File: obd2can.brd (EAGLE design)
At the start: 39.7 x 29.1 mm, 21 parts, among them Q1 16MHz, SW1 6X3.5_TACT, SW3 6X3.5_TACT, U2 SN65HVD235DR, U3 STM32F030XTSSOP20, U4 MCP1700, X1 RJ45_RIGHT_ANGLEMOLEX_95001-2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

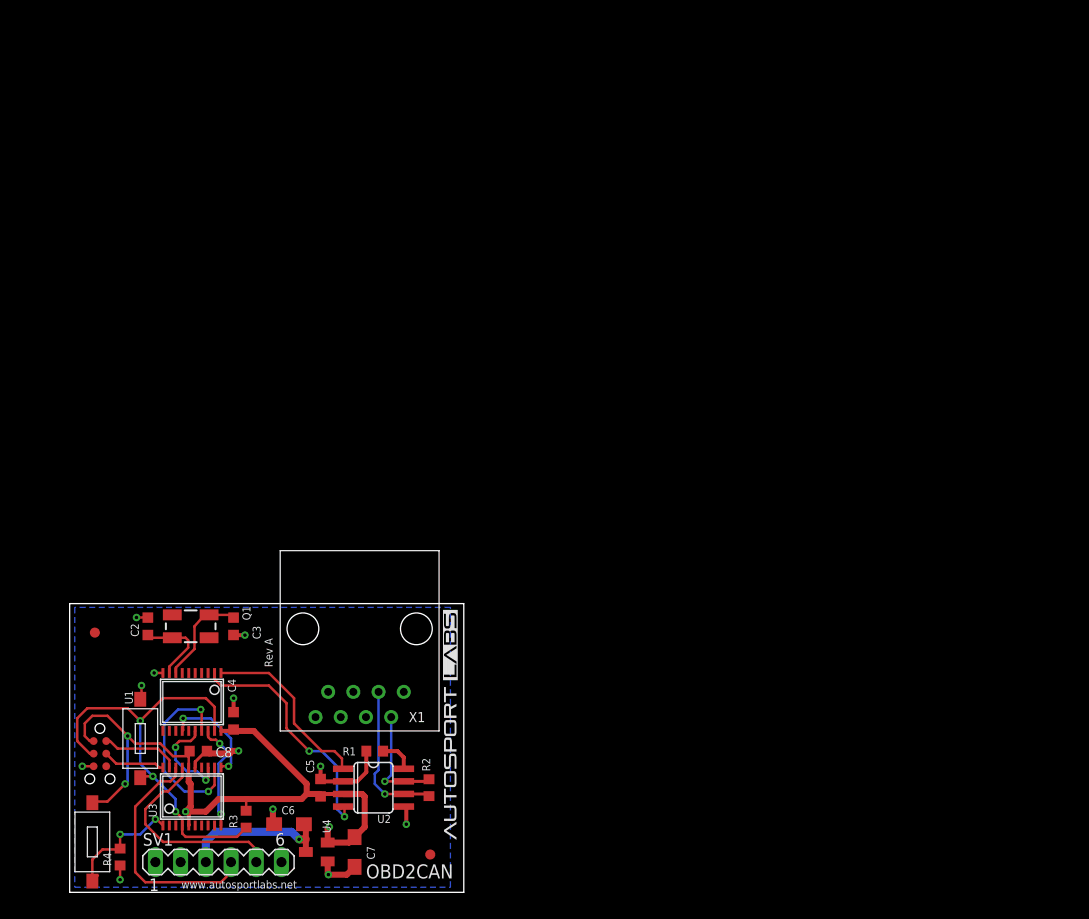
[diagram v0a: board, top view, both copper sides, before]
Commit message: OBD2CAN WIP
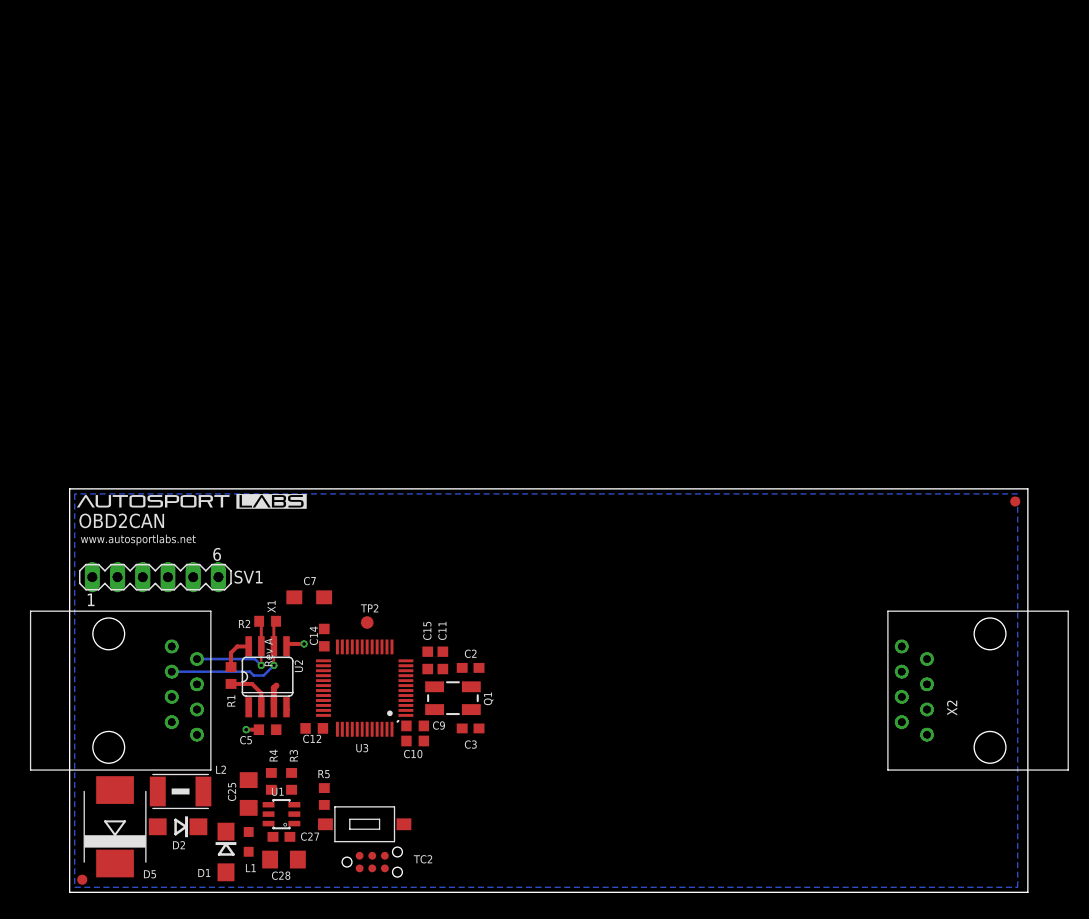
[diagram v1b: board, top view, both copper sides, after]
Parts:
- removed C4: 0.1uF, rcl:C0603K
- removed C6: 10uF, rcl:SMC_A
- removed C8: 0.1uf, rcl:C0603K
- removed SW1, SW3: 6X3.5_TACT, tactile_switch:TACT_6X3.5
- removed TC1: TC2030-IDC-NL, TagConnect:TC2030-IDC-NL
- removed U4: MCP1700, mcp1700:SOT-23
- added C10: 1uf, rcl:C0603K
- added C11: 0.01uf, rcl:C0603K
- added C12, C15: 4.7uf, rcl:C0603K
- added C14, C9: 0.1uf, rcl:C0603K
- added C25, C28: 22uF, rcl:C1206
- added C27: 10nF, rcl:C0603
- added D1: SCHOTTKY, smt_diodes:SMA
- added D2: 400V 1A, smt_diodes:SMA
- added D5: (no value), diode:SMC
- added L1: 4.7uH, rcl:L2012C
- added L2: (no value), wuerth-elektronik:1812
- added R5: 4.7K, rcl:R0603
- added SW2: 6X3.5_TACT, tactile_switch:TACT_6X3.5
- added TC2: TC2030-IDC-NL, TagConnect:TC2030-IDC-NL
- added TP2: TPB1,27, testpad:B1,27
- added X2: RJ45_RIGHT_ANGLEMOLEX_95001-2881, FCI_RJ12:RJ45_RIGHT_ANGLE_MOLEX_95001-2881
- C2, C3: value 22pF -> 33pF; device rcl:C0603K -> SparkFun:0603
- Q1: value 16MHz -> 8MHz; device SparkFun:CRYSTAL-SMD-5X3 -> SparkFun2:CRYSTAL-SMD-5X3
- R3: value 4.7K -> 16.2K 1%
- R4: value 4.7K -> 49.9K 1%
- U1: value (none) -> AP3211KTR-G1; device can:TSSOP20 -> diodes_inc:SOT-23-6
- U3: value STM32F030XTSSOP20 -> STM32F072-LQFP48; device stm32f030x:TSSOP-20 -> stm32f0:LQFP48
- moved C2 32.8 mm to (40.4, 22.6), turned to 0 degrees
- moved SV1 29.4 mm to (8.64, 31.8)
- moved Q1 27.4 mm to (38.6, 19.6), turned to 0 degrees
- moved C7 26.1 mm to (24.1, 29.7), turned to 0 degrees
- moved X1 26.0 mm to (3.94, 20.3), turned to 270 degrees
- moved C3 26.0 mm to (40.4, 16.5), turned to 180 degrees
- moved R2 23.4 mm to (19.9, 27.3), turned to 0 degrees
- moved U3 20.5 mm to (29.7, 20.6), turned to 180 degrees
- moved R4 17.0 mm to (20.3, 11.2), turned to 270 degrees
- moved R1 16.4 mm to (16.3, 21.8), turned to 90 degrees
- moved U2 15.5 mm to (19.9, 21.7), turned to 0 degrees
- moved U1 14.5 mm to (21.3, 7.87), turned to 90 degrees
- moved C5 7.91 mm to (19.9, 16.4), turned to 180 degrees
- moved R3 5.95 mm to (22.4, 11.2)
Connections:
- removed net BOOT0: R4.2, SW1.P$1, U3.1
- removed net CAN1_RX: U1.2, U2.4
- removed net CAN1_TX: U1.1, U2.1
- removed net MISO: U1.17, U3.12
- removed net MOSI: U1.16, U3.13
- removed net N$2: C3.1, Q1.1, U1.8
- removed net NPCS1: U1.18, U3.10
- removed net SPCK: U1.14, U3.11
- removed net UART1_RX: SV1.4, U3.18
- removed net UART1_TX: SV1.5, U3.17
- new net +12V: L2.2, X1.P8, X2.P8
- new net AGND: U3.8
- new net ANALOG_1_ADC: U3.10
- new net CAN_RX: U2.4, U3.32
- new net CAN_TX: U2.1, U3.33
- new net N$3: TP2.TP, U3.18
- new net N$40: C2.2, Q1.3, U3.6
- new net N$42: C3.2, Q1.1, U3.5
- new net N$5: C27.2, U1.1
- new net N$50: D2.A, L2.1
- new net N$6: C27.1, D1.C, L1.1, U1.6
- new net SAFE12V: C25.1, D2.C, D5.C, U1.4, U1.5
- new net U3: R4.1, R5.2, TC2.1
- new net USART1_RX: SV1.4, U3.31
- new net USART1_TX: SV1.5, U3.30
- new net USART2_RX: U3.13
- new net USART2_TX: U3.12
- net +5V: no longer C6.+, U4.3
- net GND: now also C10.2, C11.2, C12.2, C14.2, C15.2, C2.1, C25.2, C28.2, C3.1, C9.2, D1.A, D5.A, R3.2, SW2.P$2, TC2.5, U1.2, U3.23, U3.35, U3.44, U3.47, X2.P1; no longer C2.2, C3.2, C4.2, C6.-, C8.2, R4.1, SW3.P$2, TC1.5, U1.10, U3.15, U4.1
- net N$1: now also R3.1, R4.2, U1.3; no longer C2.1, Q1.3, U1.9
- net RESET: now also R5.1, SW2.P$1, TC2.3, U3.7; no longer R3.1, SW3.P$1, TC1.3, U1.19, U3.4
- net SWCLK: now also TC2.4, U3.37; no longer TC1.4, U3.20
- net SWDIO: now also TC2.2, U3.34; no longer TC1.2, U3.19
- net V+: now also C10.1, C11.1, C12.1, C14.1, C15.1, C28.1, C9.1, L1.2, U3.1, U3.24, U3.36, U3.48, U3.9; no longer C4.1, C8.1, R3.2, SW1.P$2, TC1.1, U1.20, U3.16, U3.5, U4.2
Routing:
- net V+: track 73.6 -> 2.29 mm, vias 4 -> 0
- net RESET: track 44.4 -> 0.00 mm, vias 3 -> 0
- net CAN1_RX: track 24.9 -> 0.00 mm, vias 2 -> 0
- net UART1_RX: track 24.3 -> 0.00 mm
- net GND: track 31.2 -> 8.15 mm, vias 12 -> 2
- net UART1_TX: track 21.1 -> 0.00 mm
- net MISO: track 19.4 -> 0.00 mm, vias 2 -> 0
- net CAN1_TX: track 18.3 -> 0.00 mm
- net +5V: track 15.8 -> 0.00 mm, vias 1 -> 0
- net BOOT0: track 12.9 -> 0.00 mm, vias 2 -> 0
- net NPCS1: track 11.0 -> 0.00 mm, vias 2 -> 0
- net SPCK: track 10.7 -> 0.00 mm, vias 2 -> 0
- net N$2: track 10.0 -> 0.00 mm
- net MOSI: track 9.68 -> 0.00 mm, vias 2 -> 0
- net N$1: track 8.41 -> 0.00 mm
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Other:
- board size 39.7 x 29.1 mm -> 96.5 x 40.6 mm

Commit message: combined designs together
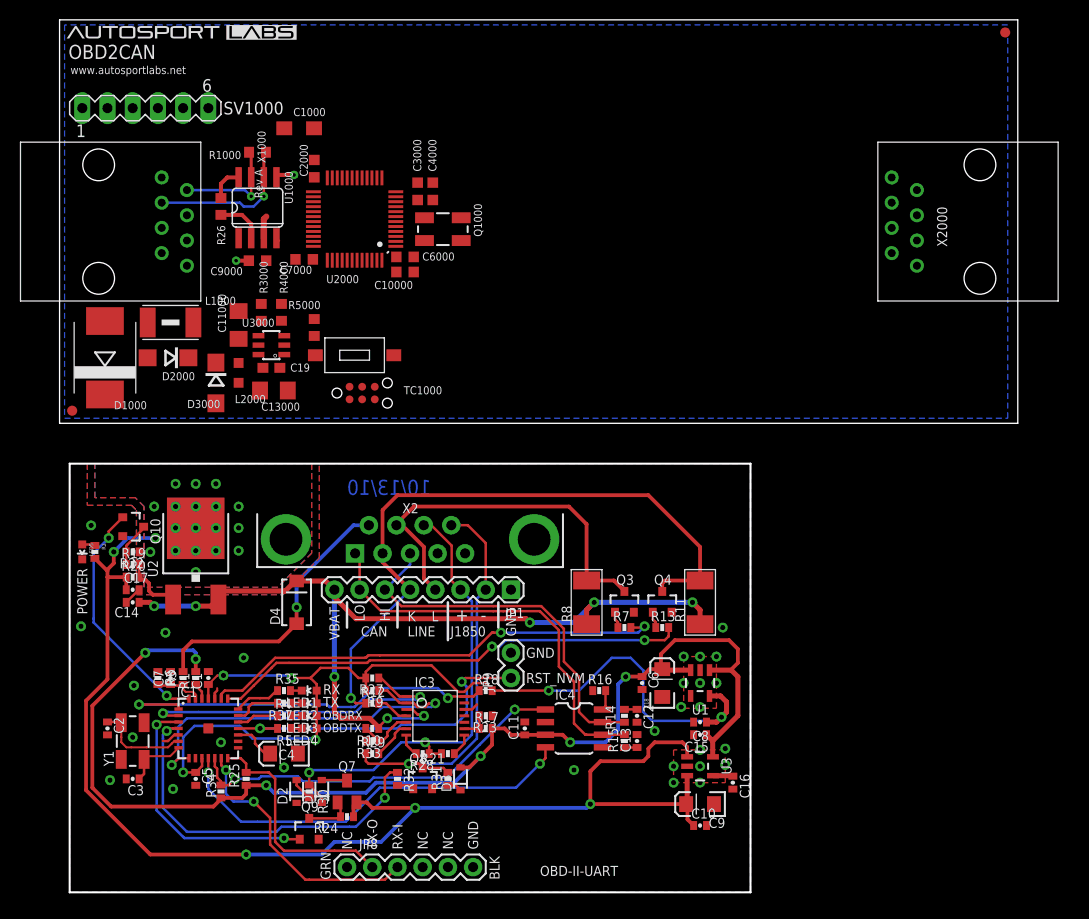
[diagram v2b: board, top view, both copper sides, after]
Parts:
- removed C25, C28: 22uF, rcl:C1206
- removed C27: 10nF, rcl:C0603
- removed D5: (no value), diode:SMC
- removed L1: 4.7uH, rcl:L2012C
- removed L2: (no value), wuerth-elektronik:1812
- removed Q1: 8MHz, SparkFun2:CRYSTAL-SMD-5X3
- removed SV1: (no value), con-lstb:MA06-1
- removed SW2: 6X3.5_TACT, tactile_switch:TACT_6X3.5
- removed TC2: TC2030-IDC-NL, TagConnect:TC2030-IDC-NL
- removed TP2: TPB1,27, testpad:B1,27
- removed X1: RJ45_RIGHT_ANGLEMOLEX_95001-2881, FCI_RJ12:RJ45_RIGHT_ANGLE_MOLEX_95001-2881
- added C1, C17, C6: 1uF, SparkFun:0402-CAP
- added C1000: 10uF, rcl:SMC_A
- added C10000: 1uf, rcl:C0603K
- added C11000, C13000: 22uF, rcl:C1206
- added C13: 560pF, SparkFun:0402-CAP
- added C16: 470pF, SparkFun:0402-CAP
- added C18: 10uF, SparkFun:EIA3216
- added C19: 10nF, rcl:C0603
- added C2000, C6000, C9000: 0.1uf, rcl:C0603K
- added C3000, C7000: 4.7uf, rcl:C0603K
- added C4: 10uF ESR<=5, SparkFun:EIA3216
- added C4000: 0.01uf, rcl:C0603K
- added C8: 4.7uF, SparkFun:0402-CAP
- added D1000: (no value), diode:SMC
- added D2000: 400V 1A, smt_diodes:SMA
- added D3: BAS16, SparkFun:SOD-323
- added D3000: SCHOTTKY, smt_diodes:SMA
- added D4: MBRA140, SparkFun:SMA-DIODE
- added IC1: SCANTOOL, SparkFun:_STN_SCANTOOL_QFN-28-S
- added IC3: LM339PWR, _stn_logic:TSSOP-14
- added IC4: MCP2551, _stn_microchip:SO-8
- added JP1: (no value), SparkFun:1X08
- added JP8: DNP, SparkFun:FTDI_BASIC
- added JP9: DNP, SparkFun:1X02
- added L1000: (no value), wuerth-elektronik:1812
- added L2000: 4.7uH, rcl:L2012C
- added LED1, LED3: YELLOW, SparkFun:LED-0603
- added LED2, LED4, LED5: RED, SparkFun:LED-0603
- added Q10, Q9: BSS138, SparkFun:SOT23-3
- added Q1000: 8MHz, SparkFun2:CRYSTAL-SMD-5X3
- added Q3, Q4, Q8: MMBT2222, SparkFun:SOT23-3
- added Q7: ZXMP6A13FTA, SparkFun:SOT23
- added R10, R12, R18, R21, R27, R28, R29, R30, R31, R33, R9: 10k, SparkFun:0402-RES
- added R1000: 120, rcl:R0603
- added R11, R8: 510 0.5W, _stn_rcl:2010
- added R13, R32, R7: 1k, SparkFun:0402-RES
- added R14, R15: 100, SparkFun:0402-RES
- added R16, R23, R25: 4.7k, SparkFun:0402-RES
- added R17: 1.2k, SparkFun:0402-RES
- added R19: 866, SparkFun:0402-RES
- added R20: 240, SparkFun:0402-RES
- added R22: 374, SparkFun:0402-RES
- added R24, R34: 1.5k, SparkFun:0402-RES
- added R26, R5000: 4.7K, rcl:R0603
- added R3000: 49.9K 1%, rcl:R0603
- added R35, R37: 330, SparkFun:0402-RES
- added R4000: 16.2K 1%, rcl:R0603
- added R6: 10K, SparkFun:0402-RES
- added SV1000: (no value), con-lstb:MA06-1
- added SW1: 6X3.5_TACT, tactile_switch:TACT_6X3.5
- added TC1000: TC2030-IDC-NL, TagConnect:TC2030-IDC-NL
- added U1000: SN65HVD235DR, can:SO08
- added U2000: STM32F072-LQFP48, stm32f0:LQFP48
- added U3000: AP3211KTR-G1, diodes_inc:SOT-23-6
- added X1000, X2000: RJ45_RIGHT_ANGLEMOLEX_95001-2881, FCI_RJ12:RJ45_RIGHT_ANGLE_MOLEX_95001-2881
- added Y1: 16MHz, SparkFun:CRYSTAL-SMD-5X3
- C10: value 1uf -> 0.1uF; device rcl:C0603K -> SparkFun:0402-CAP
- C11: value 0.01uf -> 1uF; device rcl:C0603K -> SparkFun:0402-CAP
- C12: value 4.7uf -> 560pF; device rcl:C0603K -> SparkFun:0402-CAP
- C14: value 0.1uf -> 0.1uF; device rcl:C0603K -> SparkFun:0402-CAP
- C15: value 4.7uf -> 2.2uF; device rcl:C0603K -> SparkFun:0402-CAP
- C2, C3: value 33pF -> 27pF; device SparkFun:0603 -> SparkFun:0402-CAP
- C5: value 0.1uf -> 1uF; device rcl:C0603K -> SparkFun:0402-CAP
- C7: value 10uF -> 0.1uF; device rcl:SMC_A -> SparkFun:0402-CAP
- C9: value 0.1uf -> 10uF; device rcl:C0603K -> SparkFun:EIA3216
- D1: value SCHOTTKY -> BAS16; device smt_diodes:SMA -> SparkFun:SOD-323
- D2: value 400V 1A -> BAS16; device smt_diodes:SMA -> SparkFun:SOD-323
- R1: value 4.7K -> 10k; device rcl:R0603 -> SparkFun:0402-RES
- R2: value 120 -> 1k; device rcl:R0603 -> SparkFun:0402-RES
- R3: value 16.2K 1% -> 62K; device rcl:R0603 -> SparkFun:0402-RES
- R4: value 49.9K 1% -> 330; device rcl:R0603 -> SparkFun:0402-RES
- R5: value 4.7K -> 330; device rcl:R0603 -> SparkFun:0402-RES
- U1: value AP3211KTR-G1 -> 3.3V; device diodes_inc:SOT-23-6 -> SparkFun:SOT23-5
- U2: value SN65HVD235DR -> V_REG_317DPACK; device can:SO08 -> SparkFun:V-REG_DPACK
- U3: value STM32F072-LQFP48 -> 5V Reg.; device stm32f0:LQFP48 -> SparkFun:SOT23-5
- X2: value RJ45_RIGHT_ANGLEMOLEX_95001-2881 -> Male DB9; device FCI_RJ12:RJ45_RIGHT_ANGLE_MOLEX_95001-2881 -> SparkFun:DB9_MALE
- moved X2 60.4 mm to (34.3, 35.6), turned to 0 degrees
- moved U1 44.2 mm to (63.5, 21.1), turned to 180 degrees
- moved C2 37.1 mm to (3.81, 16.5), turned to 270 degrees
- moved U3 34.7 mm to (63.5, 12.7), turned to 270 degrees
- moved C3 34.4 mm to (6.35, 11.4)
- moved C12 32.5 mm to (57.1, 17.8), turned to 270 degrees
- moved C10 29.9 mm to (63.5, 6.73)
- moved C9 29.8 mm to (63.5, 8.89), turned to 180 degrees
- moved C15 28.4 mm to (63.5, 15.9), turned to 180 degrees
- moved C14 19.6 mm to (6.35, 29.2), turned to 180 degrees
- moved R2 18.7 mm to (2.54, 34.3), turned to 270 degrees
- moved C7 16.2 mm to (10.2, 21.6), turned to 90 degrees
- moved R3 15.1 mm to (11.4, 21.6)
- moved U2 14.5 mm to (12.7, 34.3)
- moved D2 12.5 mm to (22.9, 10.2), turned to 90 degrees
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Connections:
- new net !ISO_K_TX: IC1.22, R13.2
- new net !ISO_L_TX: IC1.23, R7.2
- new net !ISO_RX: IC1.8, IC3.2, R9.1
- new net !OBD_RX_STATUS!/PGC: IC1.19, R4.1
- new net !PWR_SAVE: IC1.15
- new net !VPW_RX: IC1.1, IC3.14, R18.1
- new net 3.3V: C1.1, C5.1, C8.1, IC1.10, IC1.25, LED1.A, LED2.A, LED3.A, LED4.A, R18.2, R27.2, R9.2, U1.5
- new net 5V: C11.1, C15.1, C18.A, C6.1, D3.2, IC4.3, R1.2, R17.2, R25.1, R34.1, U1.1, U1.3, U3.5
- new net BATT_V: C7.1, IC1.27, R3.1, R6.2
- new net CAN_HI: IC4.7, JP1.6, R14.2, X2.3
- new net CAN_LO: IC4.6, JP1.7, R15.2, X2.5
- new net HOST_PRESENT: IC1.9
- new net J1850BUS+: D1.1, JP1.3, R21.1, R28.1, R30.1, X2.7
- new net J1850BUS+_TX: IC1.3, Q9.1
- new net J1850BUS-: JP1.2, Q8.3, R29.1, R31.2, X2.6
- new net J1850BUS-_TX: IC1.4, R32.1
- new net K-LINE: JP1.5, Q4.3, R11.2, R12.1, X2.4
- new net L-LINE: JP1.4, Q3.3, R8.2, X2.8
- new net N$10: C12.1, R14.1
- new net N$11: IC4.8, R16.2
- new net N$12: IC3.9, R17.1, R23.2
- new net N$13: IC3.4, R12.2
- new net N$14: D3.1, R31.1
- new net N$15: R26.2, U1000.8
- new net N$16: R3000.2, R4000.1, U3000.3
- new net N$17: C19.2, U3000.1
- new net N$18: Q7.1, Q9.3, R24.2
- new net N$19: C19.1, D3000.C, L2000.1, U3000.6
- new net N$22: Q10.3, R19.1, R22.2
- new net N$24: D2.2, R30.2
- new net N$25: Q8.1, R32.2
- new net N$26: C4.A, IC1.17
- new net N$27: C13.1, R15.1
- new net N$30: LED3.C, R4.2
- new net N$31: LED4.C, R5.1
- new net N$32: LED5.A, R2.1
- new net N$35: LED1.C, R35.2
- new net N$36: LED2.C, R37.1
- new net N$4: Q4.1, R13.1
- new net N$7: IC3.8, R21.2
- new net N$8: R19.2, R20.2, U2.1
- new net N$9: D1.2, Q7.3
- new net OSC1: C2.1, IC1.6, Y1.3
- new net OSC2: C3.1, IC1.7, Y1.1
- new net PWM/!VPW: IC1.28, Q10.1
- new net PWM_RX: IC1.2, IC3.1, R27.1
- new net RST_NVM: IC1.18, JP9.1, R5.2
- new net RX-I: IC1.13, JP8.TXO
- new net RX-STAT: IC1.21, R35.1
- new net TX-O: IC1.14, JP8.RXI, R25.2
- new net TX-STAT: IC1.20, R37.2
- new net VBAT: C14.1, D4.C, IC3.3, JP1.8, R10.1, R11.1, R8.1, U2.3
- new net VBATT_RAW: D4.A, R3.2, X2.9
- new net VCC: C10.1, C17.1, C9.A, Q7.2, R2.2, R20.1, R24.1, U2.4, U3.1, U3.3
- net +12V: now also L1000.2, X1000.P8, X2000.P8; no longer L2.2, X1.P8, X2.P8
- net +5V: now also SV1000.3; no longer SV1.3
- net AGND: now also U2000.8; no longer U3.8
- net ANALOG_1_ADC: now also U2000.10; no longer U3.10
- net CANH: now also R1000.1, U1000.7, X1000.P2; no longer R2.1, U2.7, X1.P2
- net CANL: now also R1000.2, U1000.6, X1000.P3; no longer R2.2, U2.6, X1.P3
- net CAN_RX: now also IC1.11, IC4.4, U1000.4, U2000.32; no longer U2.4, U3.32
- net CAN_TX: now also IC1.12, IC4.1, R34.2, U1000.1, U2000.33; no longer U2.1, U3.33
- net GND: now also C1.2, C1000.-, C10000.2, C11000.2, C13.2, C13000.2, C16.2, C17.2, C18.C, C2.2, C2000.2, C3.2, C3000.2, C4.C, C4000.2, C6.2, C6000.2, C7.2, C7000.2, C8.2, C9.C, C9000.2, D1000.A, D2.1, D3000.A, IC1.16, IC1.24, IC1.5, IC1.EXP, IC3.12, IC4.2, JP1.1, JP8.GND, JP9.2, LED5.C, Q10.2, Q3.2, Q4.2, Q8.2, Q9.2, R16.1, R22.1, R23.1, R26.1, R33.2, R4000.2, R6.1, SV1000.1, SW1.P$2, TC1000.5, U1000.2, U1000.5, U2000.23, U2000.35, U2000.44, U2000.47, U3.2, U3000.2, X1000.P1, X2.1, X2.2, X2000.P1; no longer C2.1, C25.2, C28.2, C3.1, C7.-, C9.2, D1.A, D5.A, R1.1, R3.2, SV1.1, SW2.P$2, TC2.5, U2.2, U2.5, U3.23, U3.35, U3.44, U3.47, X1.P1, X2.P1
- net N$1: now also IC3.7, R28.2; no longer R3.1, R4.2, U1.3
- net N$3: now also IC3.6, R29.2; no longer TP2.TP, U3.18
- net N$34: now also C16.1, U3.4; no longer R1.2, U2.8
- net N$40: now also Q1000.3, U2000.6; no longer C2.2, Q1.3, U3.6
- net N$42: now also Q1000.1, U2000.5; no longer C3.2, Q1.1, U3.5
- net N$5: now also Q3.1, R7.1; no longer C27.2, U1.1
- net N$50: now also D2000.A, L1000.1; no longer D2.A, L2.1
- net N$6: now also IC3.5, R10.2, R33.1; no longer C27.1, D1.C, L1.1, U1.6
- net RESET: now also IC1.26, R1.1, R5000.1, SW1.P$1, TC1000.3, U2000.7; no longer R5.1, SW2.P$1, TC2.3, U3.7
- net SAFE12V: now also C11000.1, D1000.C, D2000.C, U3000.4, U3000.5; no longer C25.1, D2.C, D5.C, U1.4, U1.5
- net SWCLK: now also TC1000.4, U2000.37; no longer TC2.4, U3.37
- net SWDIO: now also TC1000.2, U2000.34; no longer TC2.2, U3.34
- net U3: now also R3000.1, R5000.2, TC1000.1; no longer R4.1, R5.2, TC2.1
- net USART1_RX: now also SV1000.4, U2000.31; no longer SV1.4, U3.31
- net USART1_TX: now also SV1000.5, U2000.30; no longer SV1.5, U3.30
- net USART2_RX: now also U2000.13; no longer U3.13
- net USART2_TX: now also U2000.12; no longer U3.12
- net V+: now also C1000.+, C10000.1, C13000.1, C2000.1, C3000.1, C4000.1, C6000.1, C7000.1, C9000.1, L2000.2, U1000.3, U2000.1, U2000.24, U2000.36, U2000.48, U2000.9; no longer C10.1, C11.1, C12.1, C14.1, C15.1, C28.1, C5.1, C7.+, C9.1, L1.2, U2.3, U3.1, U3.24, U3.36, U3.48, U3.9
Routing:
- net VCC: track 0.00 -> 129.3 mm, vias 0 -> 22
- net 5V: track 0.00 -> 124.3 mm, vias 0 -> 6
- net 3.3V: track 0.00 -> 98.1 mm, vias 0 -> 6
- net VBAT: track 0.00 -> 90.1 mm, vias 0 -> 8
- net K-LINE: track 0.00 -> 67.2 mm, vias 0 -> 1
- net !ISO_K_TX: track 0.00 -> 47.9 mm, vias 0 -> 2
- net J1850BUS+: track 0.00 -> 47.7 mm, vias 0 -> 2
- net !ISO_L_TX: track 0.00 -> 47.4 mm, vias 0 -> 2
- net CAN_RX: track 0.36 -> 42.5 mm, vias 0 -> 2
- net J1850BUS-: track 0.00 -> 41.7 mm, vias 0 -> 1
- net CAN_LO: track 0.00 -> 41.3 mm
- net !VPW_RX: track 0.00 -> 40.3 mm, vias 0 -> 2
- net !ISO_RX: track 0.00 -> 39.5 mm, vias 0 -> 2
- net CAN_TX: track 0.00 -> 39.3 mm, vias 0 -> 2
- net L-LINE: track 0.00 -> 39.2 mm
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- added copper zone on layer 1, net GND
- added copper zone on layer 1, net VCC
- added copper zone on layer 16, net VCC
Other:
- board size 96.5 x 40.6 mm -> 96.5 x 87.9 mm
- board text added: "+"
- board text added: "-"
- board text added: "10/13/10"
- board text added: "BLK"
- board text added: "CAN"
- board text added: "GND"
- board text added: "GRN"
- board text added: "HI"
- board text added: "J1850"
- board text added: "K"
- board text added: "L"
- board text added: "LINE"
- board text added: "LO"
- board text added: "NC"
- board text added: "OBD-II-UART"
- board text added: "OBDRX"
- board text added: "OBDTX"
- board text added: "POWER"
- board text added: "RST_NVM"
- board text added: "RX"
- board text added: "RX-I"
- board text added: "TX"
- board text added: "TX-O"
- board text added: "VBAT"
